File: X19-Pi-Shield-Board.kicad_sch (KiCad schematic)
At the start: 32 parts, among them J1 Raspberry_Pi_5, J3 Conn_01x02, J4 Conn_01x06, J5 Conn_01x04, J6 Conn_01x03, J7 Conn_01x05_Pin, J8 Conn_01x02, U2 BME280

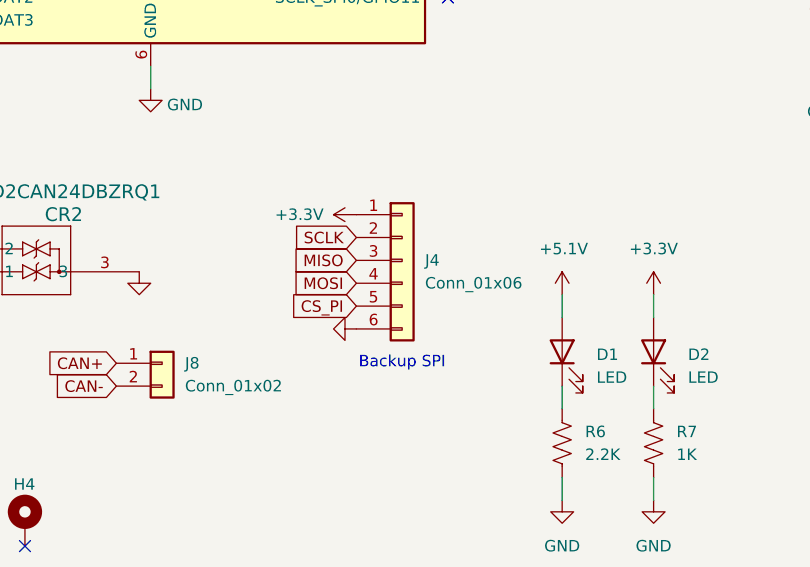
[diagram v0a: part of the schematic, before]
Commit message: footprints COMPLETELY DONE
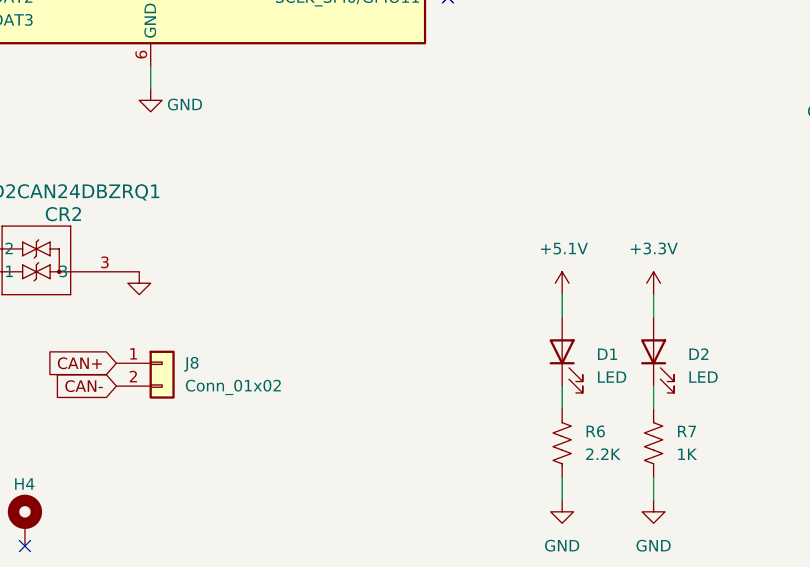
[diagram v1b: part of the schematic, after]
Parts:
- removed J4: Conn_01x06, Connector_PinHeader_2.54mm:PinHeader_1x06_P2.54mm_Vertical, symbol Connector_Generic:Conn_01x06
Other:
- note removed: "Backup SPI"
